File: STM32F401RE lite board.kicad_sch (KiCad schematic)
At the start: 45 parts, among them J1 USB_B_Micro, J2 Conn_01x04_Pin, J3 Conn_01x05_Pin, J4 Conn_01x04_Pin, J5 Conn_01x05_Pin, J7 Conn_01x19_Pin, J8 Conn_01x22_Pin, SW1 SW_Push, SW2 SW_SPDT, U1 USBLC6-2SC6, U2 LD3985M33R_SOT23, U3 STM32F401RETx, Y1 8MHz(16pF)

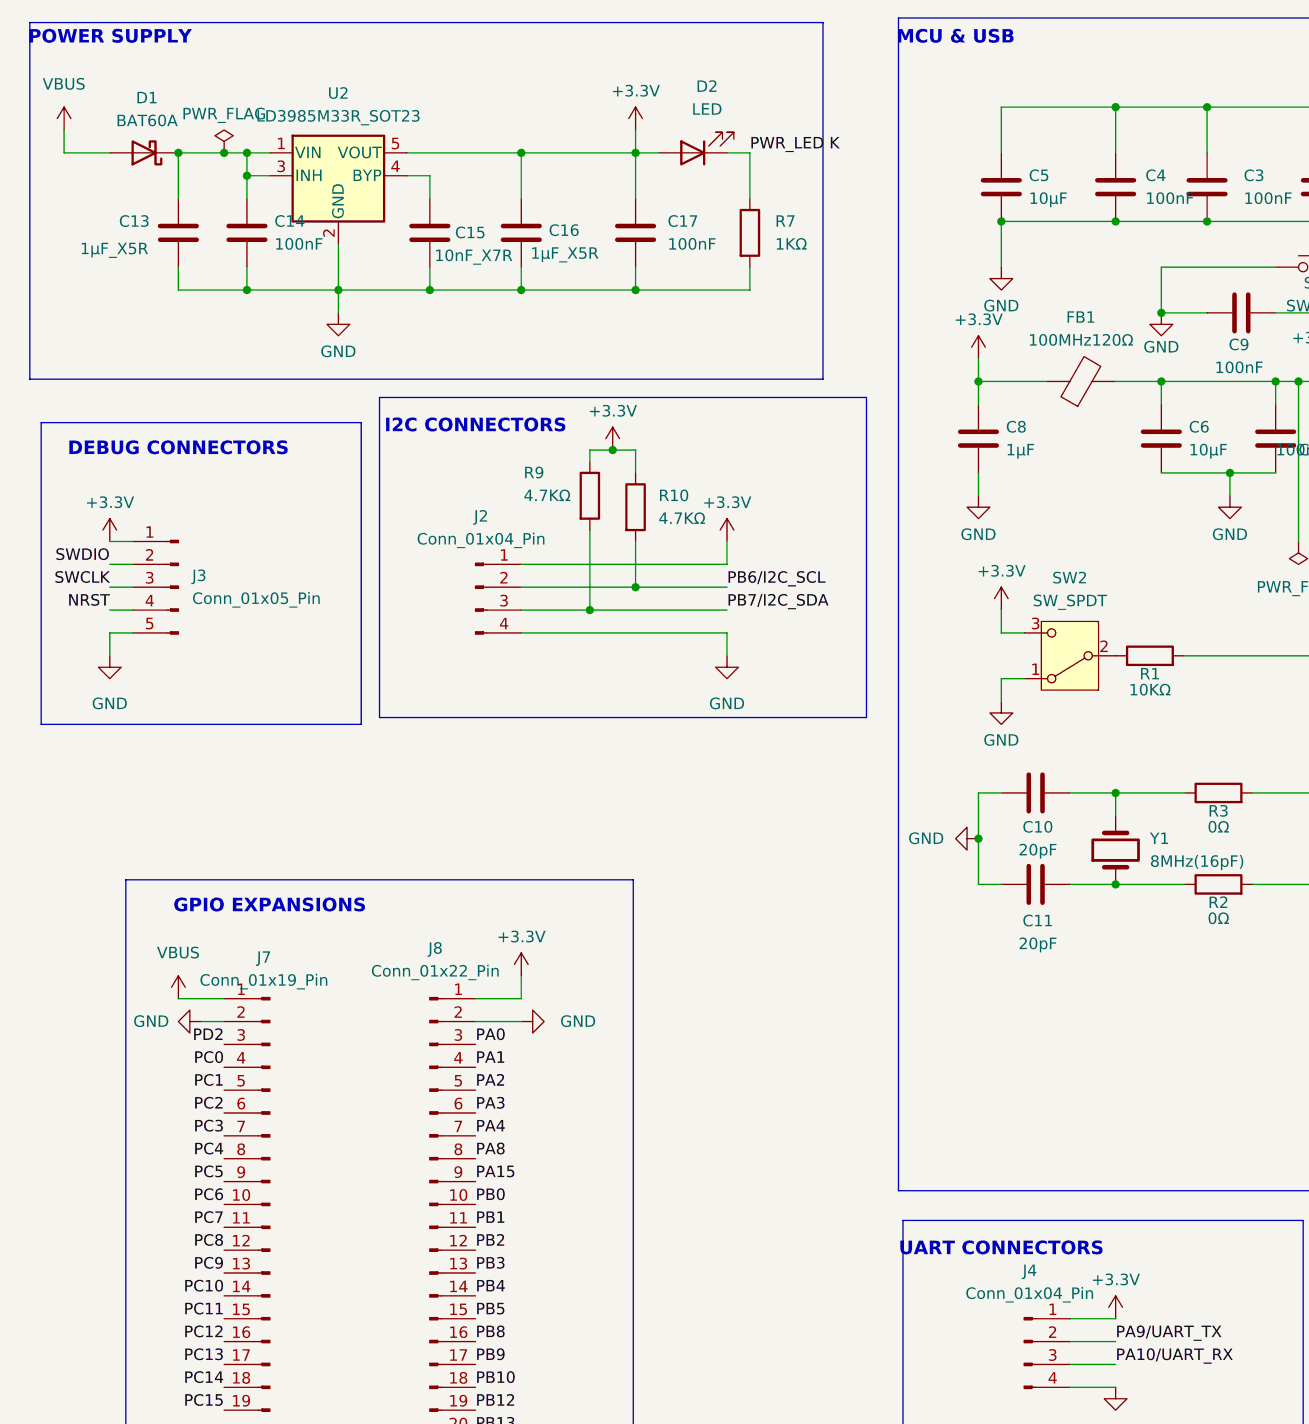
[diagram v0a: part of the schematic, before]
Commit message: C4
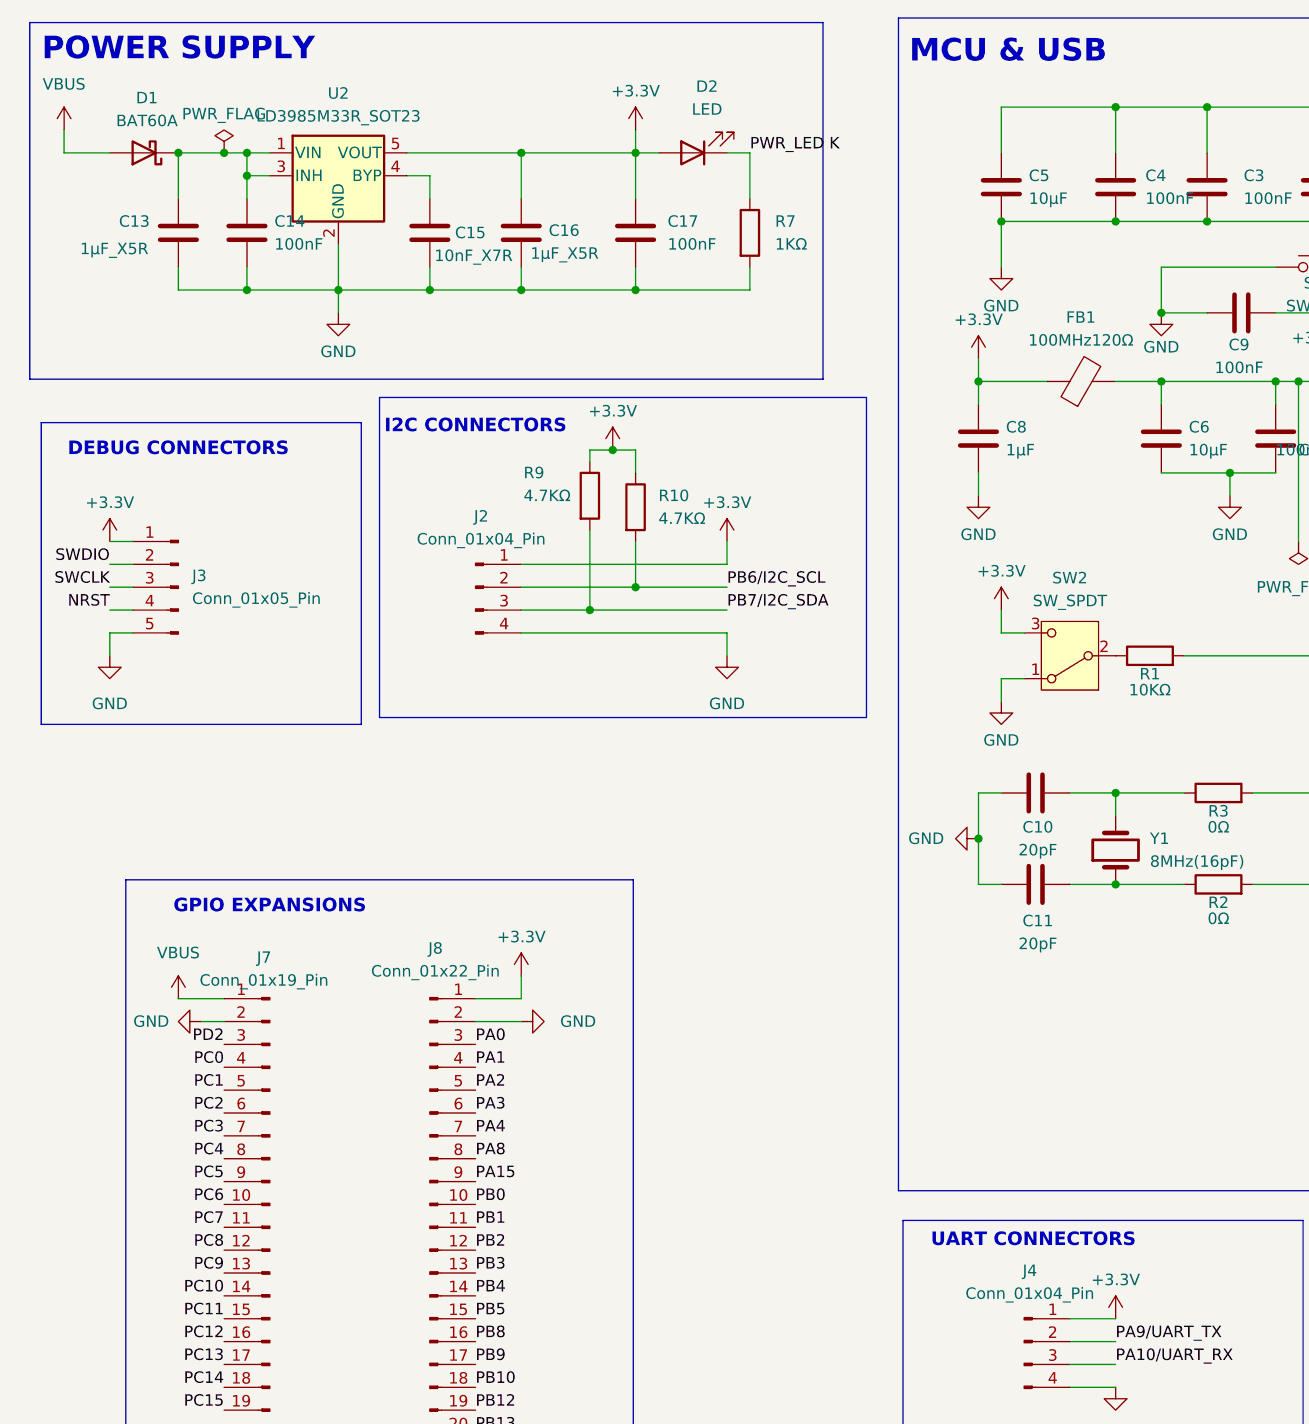
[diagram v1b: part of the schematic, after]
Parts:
- C1, C10, C11, C12, C13, C15, C16, C17, C2, C3, C4, C7, C8: footprint (none) -> Capacitor_SMD:C_0402_1005Metric
- C14, C18, C5, C6, C9: footprint (none) -> Capacitor_SMD:C_0603_1608Metric
- D2, D3: footprint (none) -> LED_SMD:LED_0603_1608Metric
- FB1: footprint (none) -> Inductor_SMD:L_0603_1608Metric
- J1: footprint (none) -> Connector_USB:USB_Micro-B_Molex-105017-0001
- Y1: footprint (none) -> Crystal:Crystal_SMD_HC49-SD
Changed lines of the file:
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@@
 	(text "POWER SUPPLY"
 		(exclude_from_sim no)
-		(at 22.86 15.24 0)
+		(at 30.48 16.51 0)
 		(effects
 			(font
-				(size 1.5 1.5)
+				(size 2.5 2.5)
 				(thickness 0.3)
 				(bold yes)
@@
 	(text "MCU & USB"
 		(exclude_from_sim no)
-		(at 116.84 15.24 0)
+		(at 122.682 16.764 0)
 		(effects
 			(font
-				(size 1.5 1.5)
+				(size 2.5 2.5)
 				(thickness 0.3)
 				(bold yes)
@@
 	(text "UART CONNECTORS\n"
 		(exclude_from_sim no)
-		(at 121.92 149.86 0)
+		(at 125.476 148.844 0)
 		(effects
 			(font
@@
 			)
 		)
-		(property "Footprint" ""
+		(property "Footprint" "Capacitor_SMD:C_0402_1005Metric"
 			(at 31.4452 40.64 0)
 			(effects
@@
 			)
 		)
-		(property "Footprint" ""
+		(property "Footprint" "Capacitor_SMD:C_0402_1005Metric"
 			(at 82.2452 40.64 0)
 			(effects
@@
 			)
 		)
-		(property "Footprint" ""
+		(property "Footprint" "LED_SMD:LED_0603_1608Metric"
 			(at 87.63 27.94 0)
 			(effects
@@
 			)
 		)
-		(property "Footprint" ""
+		(property "Footprint" "Capacitor_SMD:C_0402_1005Metric"
 			(at 145.7452 35.56 0)
 			(effects
@@
 			)
 		)
-		(property "Footprint" ""
+		(property "Footprint" "Capacitor_SMD:C_0603_1608Metric"
 			(at 152.4 44.7548 0)
 			(effects
@@
 			)
 		)
-		(property "Footprint" ""
+		(property "Footprint" "Capacitor_SMD:C_0402_1005Metric"
 			(at 135.5852 35.56 0)
 			(effects
@@
 			)
 		)
-		(property "Footprint" ""
+		(property "Footprint" "Crystal:Crystal_SMD_HC49-SD"
 			(at 134.62 105.41 0)
 			(effects
@@
 			)
 		)
-		(property "Footprint" ""
+		(property "Footprint" "Capacitor_SMD:C_0402_1005Metric"
 			(at 69.5452 40.64 0)
 			(effects
@@
 			)
 		)
-		(property "Footprint" ""
+		(property "Footprint" "Connector_USB:USB_Micro-B_Molex-105017-0001"
 			(at 245.11 72.39 0)
 			(effects
@@
 			)
 		)
-		(property "Footprint" ""
+		(property "Footprint" "Capacitor_SMD:C_0402_1005Metric"
 			(at 153.3652 63.5 0)
 			(effects
@@
 			)
 		)
-		(property "Footprint" ""
+		(property "Footprint" "Capacitor_SMD:C_0603_1608Metric"
 			(at 163.5252 124.46 0)
 			(effects
@@
 			)
 		)
-		(property "Footprint" ""
+		(property "Footprint" "Capacitor_SMD:C_0402_1005Metric"
 			(at 129.54 98.0948 0)
 			(effects
@@
 			)
 		)
-		(property "Footprint" ""
+		(property "Footprint" "Inductor_SMD:L_0603_1608Metric"
 			(at 130.81 55.118 90)
 			(effects
@@
 			)
 		)
-		(property "Footprint" ""
+		(property "Footprint" "Capacitor_SMD:C_0402_1005Metric"
 			(at 168.6052 35.56 0)
 			(effects
@@
 			)
 		)
-		(property "Footprint" ""
+		(property "Footprint" "Capacitor_SMD:C_0402_1005Metric"
 			(at 275.2852 66.04 0)
 			(effects
@@
 			)
 		)
-		(property "Footprint" ""
+		(property "Footprint" "LED_SMD:LED_0603_1608Metric"
 			(at 41.91 185.42 0)
 			(effects
@@
 			)
 		)
-		(property "Footprint" ""
+		(property "Footprint" "Capacitor_SMD:C_0402_1005Metric"
 			(at 158.4452 35.56 0)
 			(effects
@@
 			)
 		)
-		(property "Footprint" ""
+		(property "Footprint" "Capacitor_SMD:C_0402_1005Metric"
 			(at 59.3852 40.64 0)
 			(effects
@@
 			)
 		)
-		(property "Footprint" ""
+		(property "Footprint" "Capacitor_SMD:C_0402_1005Metric"
 			(at 129.54 108.2548 0)
 			(effects
@@
 			)
 		)
-		(property "Footprint" ""
+		(property "Footprint" "Capacitor_SMD:C_0603_1608Metric"
 			(at 122.8852 35.56 0)
 			(effects
@@
 			)
 		)
-		(property "Footprint" ""
+		(property "Footprint" "Capacitor_SMD:C_0603_1608Metric"
 			(at 140.6652 63.5 0)
 			(effects
@@
 			)
 		)
-		(property "Footprint" ""
+		(property "Footprint" "Capacitor_SMD:C_0402_1005Metric"
 			(at 120.3452 63.5 0)
 			(effects
@@
 			)
 		)
-		(property "Footprint" ""
+		(property "Footprint" "Capacitor_SMD:C_0603_1608Metric"
 			(at 39.0652 40.64 0)
 			(effects

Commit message: C5
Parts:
- J2, J4: footprint (none) -> Connector_PinHeader_2.54mm:PinHeader_1x04_P2.54mm_Vertical
- J3, J5: footprint (none) -> Connector_PinHeader_2.54mm:PinHeader_1x05_P2.54mm_Vertical
- J7: footprint (none) -> Connector_PinHeader_2.54mm:PinHeader_1x19_P2.54mm_Vertical
- J8: footprint (none) -> Connector_PinHeader_2.54mm:PinHeader_1x22_P2.54mm_Vertical
- R1, R10, R2, R3, R4, R5, R6, R7, R8, R9: footprint (none) -> Resistor_SMD:R_0402_1005Metric
- SW1: footprint (none) -> Button_Switch_SMD:SW_Push_1TS009xxxx-xxxx-xxxx_6x6x5mm
- SW2: footprint (none) -> Button_Switch_SMD:SW_SPST_B3U-1000P
- Y1: footprint Crystal:Crystal_SMD_HC49-SD -> Crystal:Crystal_HC49-4H_Vertical
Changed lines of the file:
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@@
 			)
 		)
-		(property "Footprint" ""
+		(property "Footprint" "Connector_PinHeader_2.54mm:PinHeader_1x04_P2.54mm_Vertical"
 			(at 63.5 76.2 0)
 			(effects
@@
 			)
 		)
-		(property "Footprint" ""
+		(property "Footprint" "Resistor_SMD:R_0402_1005Metric"
 			(at 222.25 71.882 90)
 			(effects
@@
 			)
 		)
-		(property "Footprint" ""
+		(property "Footprint" "Connector_PinHeader_2.54mm:PinHeader_1x22_P2.54mm_Vertical"
 			(at 58.42 147.32 0)
 			(effects
@@
 			)
 		)
-		(property "Footprint" ""
+		(property "Footprint" "Connector_PinHeader_2.54mm:PinHeader_1x04_P2.54mm_Vertical"
 			(at 124.46 160.02 0)
 			(effects
@@
 			)
 		)
-		(property "Footprint" ""
+		(property "Footprint" "Connector_PinHeader_2.54mm:PinHeader_1x19_P2.54mm_Vertical"
 			(at 40.64 144.78 0)
 			(effects
@@
 			)
 		)
-		(property "Footprint" "Crystal:Crystal_SMD_HC49-SD"
+		(property "Footprint" "Crystal:Crystal_HC49-4H_Vertical"
 			(at 134.62 105.41 0)
 			(effects
@@
 			)
 		)
-		(property "Footprint" ""
+		(property "Footprint" "Connector_PinHeader_2.54mm:PinHeader_1x05_P2.54mm_Vertical"
 			(at 30.48 76.2 0)
 			(effects
@@
 			)
 		)
-		(property "Footprint" ""
+		(property "Footprint" "Resistor_SMD:R_0402_1005Metric"
 			(at 92.202 36.83 90)
 			(effects
@@
 			)
 		)
-		(property "Footprint" ""
+		(property "Footprint" "Resistor_SMD:R_0402_1005Metric"
 			(at 265.938 64.77 90)
 			(effects
@@
 			)
 		)
-		(property "Footprint" ""
+		(property "Footprint" "Button_Switch_SMD:SW_Push_1TS009xxxx-xxxx-xxxx_6x6x5mm"
 			(at 157.48 35.56 0)
 			(effects
@@
 			)
 		)
-		(property "Footprint" ""
+		(property "Footprint" "Resistor_SMD:R_0402_1005Metric"
 			(at 54.61 187.198 90)
 			(effects
@@
 			)
 		)
-		(property "Footprint" ""
+		(property "Footprint" "Connector_PinHeader_2.54mm:PinHeader_1x05_P2.54mm_Vertical"
 			(at 134.62 185.42 0)
 			(effects
@@
 			)
 		)
-		(property "Footprint" ""
+		(property "Footprint" "Resistor_SMD:R_0402_1005Metric"
 			(at 222.25 69.342 90)
 			(effects
@@
 			)
 		)
-		(property "Footprint" ""
+		(property "Footprint" "Resistor_SMD:R_0402_1005Metric"
 			(at 79.502 67.31 90)
 			(effects
@@
 			)
 		)
-		(property "Footprint" ""
+		(property "Footprint" "Button_Switch_SMD:SW_SPST_B3U-1000P"
 			(at 129.54 83.82 0)
 			(effects
@@
 			)
 		)
-		(property "Footprint" ""
+		(property "Footprint" "Resistor_SMD:R_0402_1005Metric"
 			(at 138.43 85.598 90)
 			(effects
@@
 			)
 		)
-		(property "Footprint" ""
+		(property "Footprint" "Resistor_SMD:R_0402_1005Metric"
 			(at 146.05 100.838 90)
 			(effects
@@
 			)
 		)
-		(property "Footprint" ""
+		(property "Footprint" "Resistor_SMD:R_0402_1005Metric"
 			(at 74.422 66.04 90)
 			(effects
@@
 			)
 		)
-		(property "Footprint" ""
+		(property "Footprint" "Resistor_SMD:R_0402_1005Metric"
 			(at 146.05 110.998 90)
 			(effects

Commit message: C6
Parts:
- SW2: footprint Button_Switch_SMD:SW_SPST_B3U-1000P -> Button_Switch_SMD:SW_SPDT_CK_JS102011SAQN
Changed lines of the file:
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@@
 			)
 		)
-		(property "Footprint" "Button_Switch_SMD:SW_SPST_B3U-1000P"
+		(property "Footprint" "Button_Switch_SMD:SW_SPDT_CK_JS102011SAQN"
 			(at 129.54 83.82 0)
 			(effects
